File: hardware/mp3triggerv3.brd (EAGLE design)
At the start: 160 x 100 mm, 0 parts

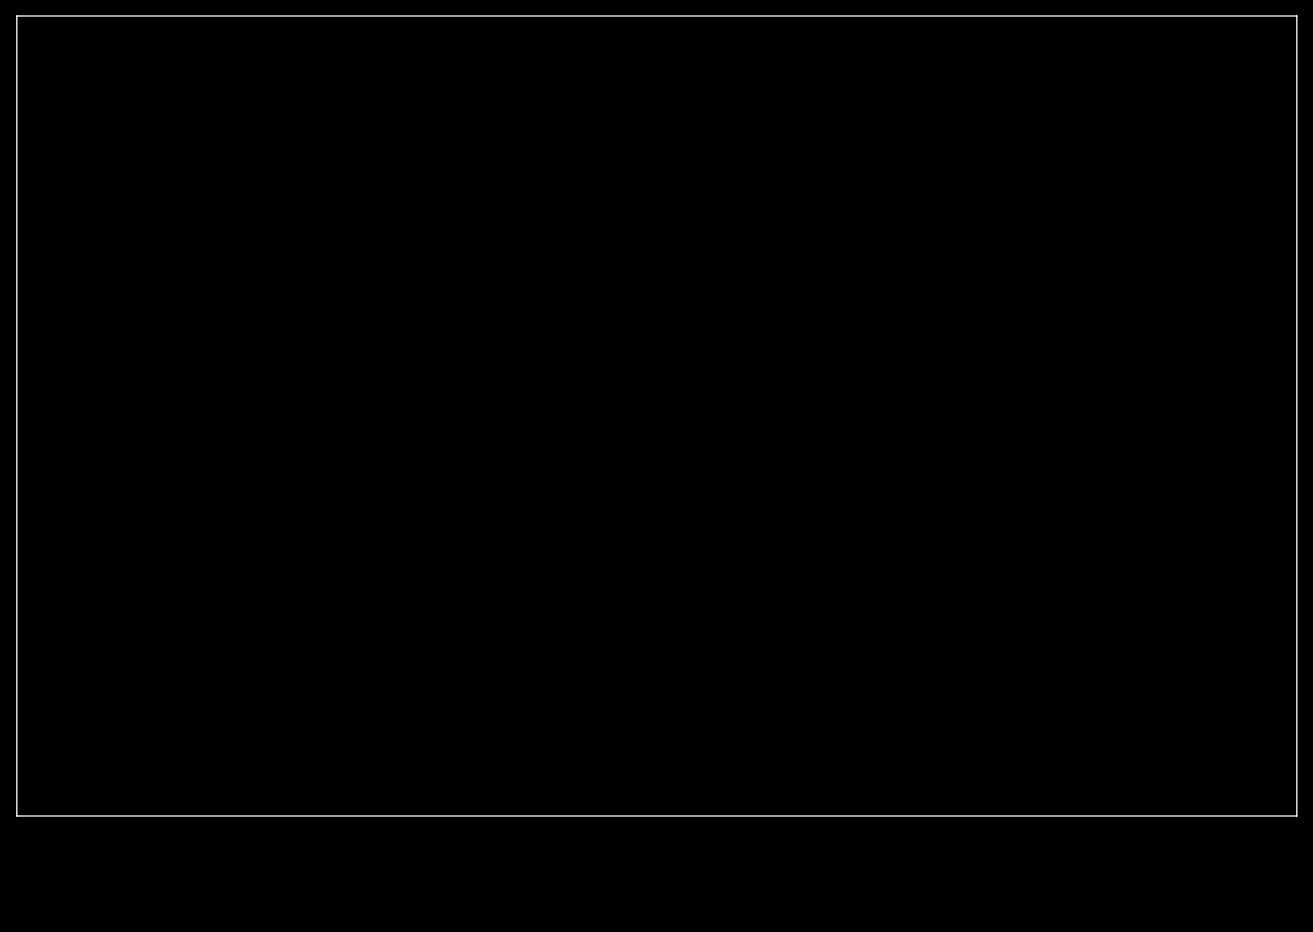
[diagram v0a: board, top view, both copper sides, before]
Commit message: added Jamie's project files
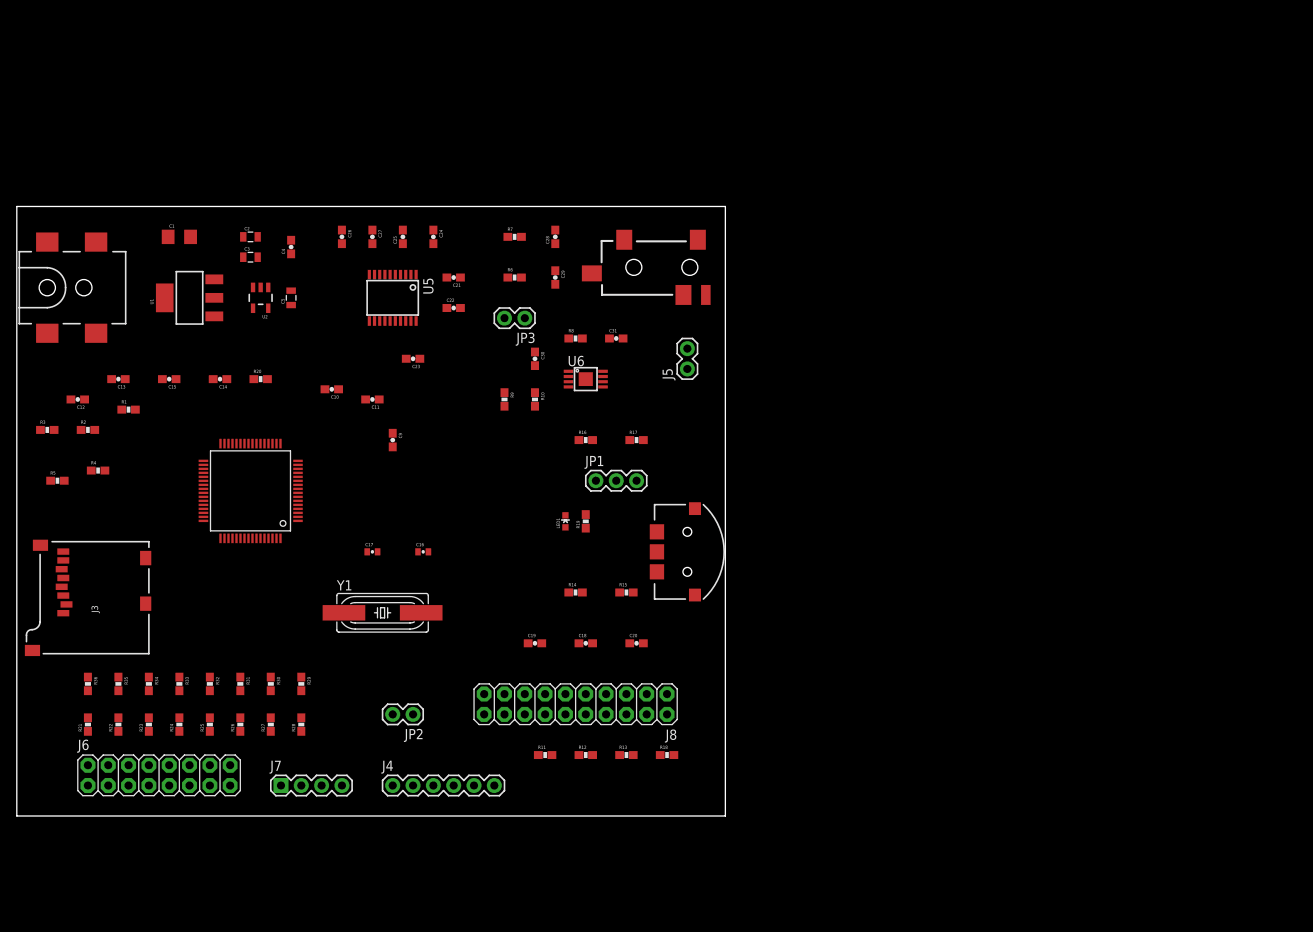
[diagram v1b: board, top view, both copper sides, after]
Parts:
- added C1: 10uF, SparkFun-Capacitors:1206
- added C10, C13, C15, C18, C19, C21, C22, C23, C24, C25, C26, C4, C9: 0.1uF, SparkFun-Capacitors:0603-CAP
- added C11, C30, C31: 1uF, SparkFun-Capacitors:0603-CAP
- added C12: 4.7uF, SparkFun-Capacitors:0603-CAP
- added C14, C20: 2.2uF, SparkFun-Capacitors:0603-CAP
- added C16, C17: 33pF, SparkFun-Capacitors:0402-CAP
- added C2: 10uF, SparkFun-Capacitors:0805
- added C27: 10uF, SparkFun-Capacitors:0603-CAP
- added C28, C29: 2200pF, SparkFun-Capacitors:0603-CAP
- added C3, C5: 2.2uF, SparkFun-Capacitors:0805
- added J1: 5.5x2.1mm Barrel, SparkFun-Connectors:POWER_JACK_SMD
- added J2: (no value), SparkFun-Connectors:AUDIO-JACK-3.5MM-SMD
- added J3: USD-SOCKETNEW, robertsonics:MICRO-SD-SOCKET-PP
- added J4: (no value), SparkFun-Connectors:1X06
- added J5, JP2, JP3: (no value), SparkFun-Connectors:1X02
- added J6: M08X2, SparkFun-Connectors:2X8
- added J7: (no value), SparkFun-Connectors:1X04
- added J8: M10X2, SparkFun-Connectors:2X10
- added JP1: (no value), SparkFun-Connectors:1X03
- added LED1: (no value), SparkFun-LED:LED-0603
- added R1, R2, R3, R4, R5: 47K, SparkFun-Passives:0603-RES
- added R10, R9: 22K, SparkFun-Passives:0603-RES
- added R11, R12, R13, R14, R15, R16, R17, R18, R20, R29, R30, R31, R32, R33, R34, R35, R36, R8: 10K, SparkFun-Passives:0603-RES
- added R19: 330, SparkFun-Passives:0603-RES
- added R21, R22, R23, R24, R25, R26, R27, R28: 100, SparkFun-Passives:0603-RES
- added R6, R7: 470, SparkFun-Passives:0603-RES
- added S1: NAV_SWITCHSMD, SparkFun-Electromechanical:NAV_SWITCH
- added U1: NCP1117, SparkFun-PowerIC:SOT223
- added U2: MIC5323-3.3, SparkFun-PowerIC:SOT23-5
- added U4: STM32F405RG, robertsonics:TQFP-10X10-64
- added U5: PCM5100, robertsonics:PW_R-PDSO-G20
- added U6: LM4990, robertsonics:S-PDSO-G08
- added Y1: 8MHz, SparkFun-FreqCtrl:HC49UP
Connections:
- new net +5V: C2.1, C3.1, C31.2, J7.4, JP2.2, U1.2, U1.4, U2.1, U2.3, U6.6
- new net AMPENA: R8.2, U4.P$11, U6.1
- new net AMPIN: JP3.2, R9.1
- new net BOOT0: JP1.2, U4.P$60
- new net DEMP: U4.P$10, U5.10
- new net FILTER: U4.P$9, U5.11
- new net GND: C1.2, C10.2, C11.2, C12.2, C13.2, C14.2, C15.2, C16.1, C17.1, C18.2, C19.2, C2.2, C20.2, C21.1, C22.2, C23.1, C25.2, C26.1, C27.1, C28.1, C29.1, C3.2, C30.1, C31.1, C4.2, C5.2, J1.GND, J1.P$4, J2.SLEEVE, J3.6, J3.CD2, J3.GND1, J3.GND3, J4.1, J6.1, J6.11, J6.13, J6.15, J6.3, J6.5, J6.7, J6.9, J7.1, J8.10, J8.12, J8.14, J8.16, J8.18, J8.20, J8.4, J8.6, J8.8, R11.1, R12.1, R13.1, R16.2, R20.2, R8.1, S1.C, U1.1, U2.2, U4.P$12, U4.P$18, U4.P$63, U5.16, U5.19, U5.3, U5.9, U6.7
- new net I2S_BCLK: U4.P$34, U5.13
- new net I2S_DOUT: U4.P$36, U5.14
- new net I2S_LRCK: U4.P$33, U5.15
- new net I2S_MCLK: U4.P$37, U5.12
- new net JTCK: J8.9, U4.P$49
- new net JTDI: J8.5, U4.P$50
- new net JTDO: J8.13, U4.P$55
- new net JTMS: J8.7, U4.P$46
- new net JTRST: J8.3, U4.P$56
- new net LED1: LED1.C, U4.P$24
- new net LOUTL: C28.2, J2.TIP, JP3.1, R7.2
- new net LOUTR: C29.2, J2.RING, R6.2
- new net MUTE: U4.P$8, U5.17
- new net N$10: JP1.3, R17.2
- new net N$11: LED1.A, R19.2
- new net N$12: R20.1, U4.P$28
- new net N$13: J8.19, R11.2
- new net N$14: C23.2, U5.18
- new net N$15: R6.1, U5.7
- new net N$16: C24.2, U5.2
- new net N$17: C24.1, U5.4
- new net N$18: C25.1, U5.5
- new net N$19: R7.1, U5.6
- new net N$2: C4.1, U2.4
- new net N$20: C30.2, U6.2, U6.3
- new net N$21: J8.17, R12.2
- new net N$22: J8.11, R13.2
- new net N$23: J6.2, R21.1, R36.1
- new net N$24: J6.4, R22.1, R35.1
- new net N$25: J6.6, R23.1, R34.1
- new net N$26: J6.8, R24.1, R33.1
- new net N$27: J6.10, R25.1, R32.1
- new net N$28: J6.12, R26.1, R31.1
- new net N$29: R10.1, R9.2, U6.4
- new net N$3: C9.2, U4.P$1
- new net N$30: J6.14, R27.1, R30.1
- new net N$31: J6.16, R28.1, R29.1
- new net N$32: J4.3, JP2.1
- new net N$4: C14.1, U4.P$31
- new net N$5: C16.2, U4.P$5, Y1.2
- new net N$6: C17.2, U4.P$6, Y1.1
- new net N$7: JP1.1, R16.1
- new net N$8: C20.1, U4.P$47
- new net N$9: J4.4, R15.2
- new net NAV1: S1.1, U4.P$2
- new net NAV2: S1.2, U4.P$4
- new net NAVT: S1.T, U4.P$3
- new net NRST: J8.15, R18.1, U4.P$7
- new net PLAYOUT: J7.2, U4.P$25
- new net RXD: R14.1, R15.1, U4.P$43
- new net SD_CD: J3.CD1, U4.P$26
- new net SD_CK: J3.5, U4.P$53
- new net SD_CMD: J3.3, R3.1, U4.P$54
- new net SD_D0: J3.7, R2.1, U4.P$39
- new net SD_D1: J3.8, R1.1, U4.P$40
- new net SD_D2: J3.1, R5.1, U4.P$51
- new net SD_D3: J3.2, R4.1, U4.P$52
- new net SPKR+: J5.2, U6.8
- new net SPKR-: J5.1, R10.2, U6.5
- new net TRIG00: R21.2, U4.P$14
- new net TRIG01: R22.2, U4.P$15
- new net TRIG02: R23.2, U4.P$16
- new net TRIG03: R24.2, U4.P$17
- new net TRIG04: R25.2, U4.P$20
- new net TRIG05: R26.2, U4.P$21
- new net TRIG06: R27.2, U4.P$22
- new net TRIG07: R28.2, U4.P$23
- new net TXD: J4.5, U4.P$42
- new net VCC: C10.1, C11.1, C12.1, C13.1, C15.1, C18.1, C19.1, C21.2, C22.1, C26.2, C27.2, C5.1, C9.1, J3.4, J7.3, J8.1, J8.2, R1.2, R14.2, R17.1, R18.2, R19.1, R2.2, R29.2, R3.2, R30.2, R31.2, R32.2, R33.2, R34.2, R35.2, R36.2, R4.2, R5.2, U2.5, U4.P$13, U4.P$19, U4.P$32, U4.P$48, U4.P$64, U5.1, U5.20, U5.8
- new net VIN_9V: C1.1, J1.VIN0, U1.3
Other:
- board size 160 x 100 mm -> 88.6 x 76.2 mm

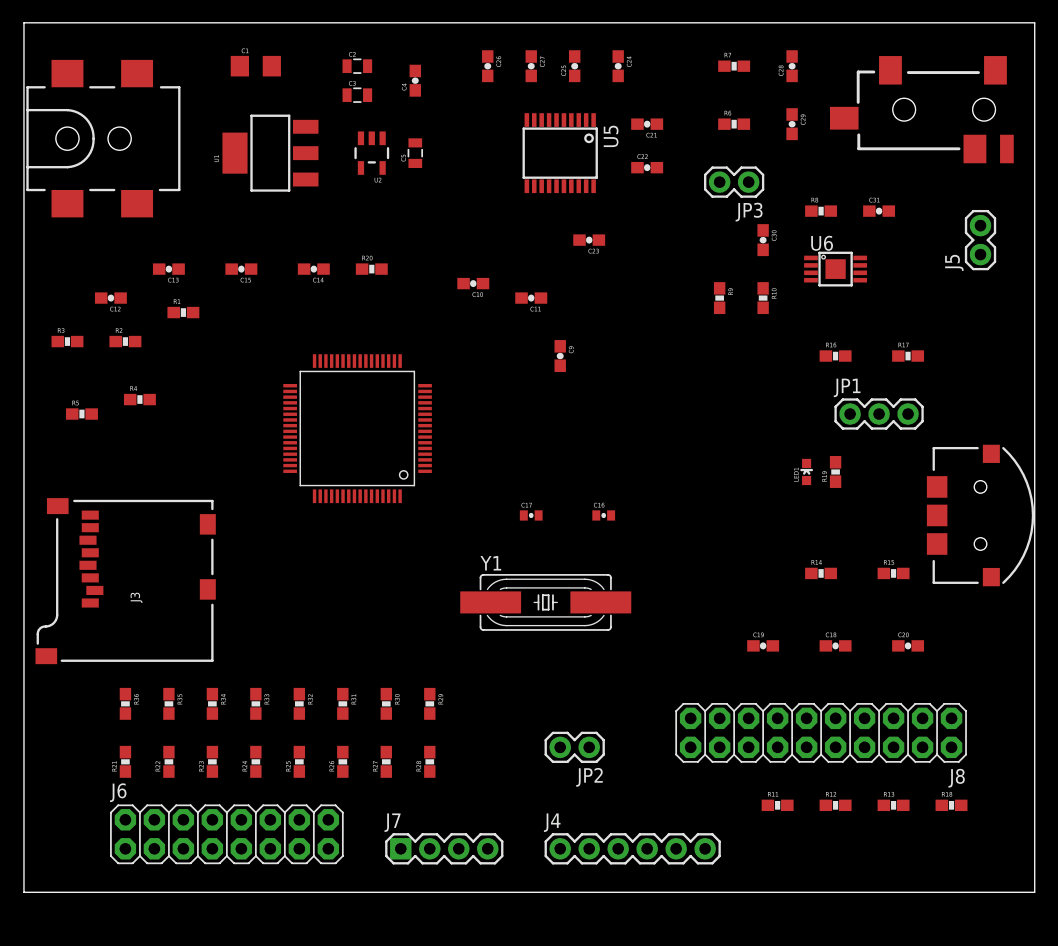
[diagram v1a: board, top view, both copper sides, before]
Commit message: v010
files sent to Jamie
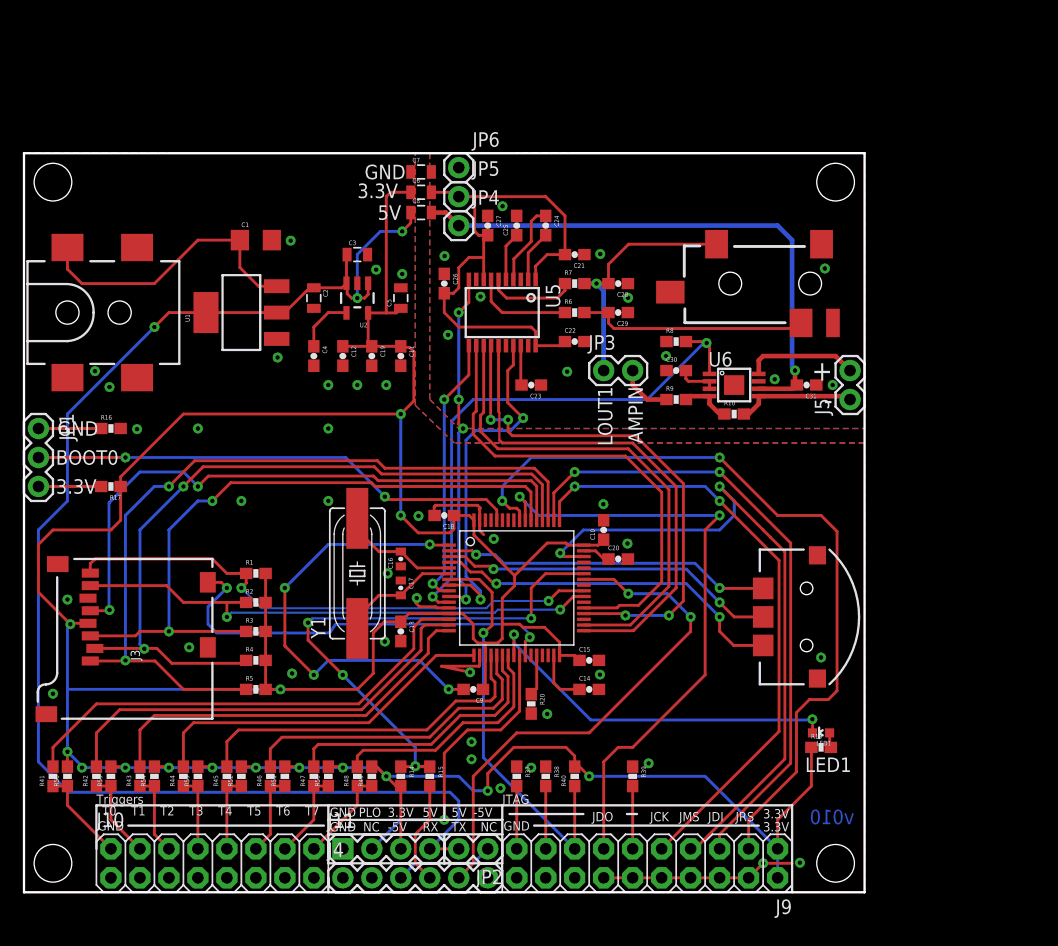
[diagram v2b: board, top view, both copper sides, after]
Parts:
- removed J6: M08X2, SparkFun-Connectors:2X8
- removed J7: (no value), SparkFun-Connectors:1X04
- removed J8: M10X2, SparkFun-Connectors:2X10
- removed R11, R12, R13, R18, R29, R30, R31, R32, R33, R34, R35, R36: 10K, SparkFun-Passives:0603-RES
- removed R21, R22, R23, R24, R25, R26, R27, R28: 100, SparkFun-Passives:0603-RES
- added C6: 3.3V jumper, SparkFun-Capacitors:0805
- added C7: GND jumper, SparkFun-Capacitors:0805
- added C8: 5V jumper, SparkFun-Capacitors:0805
- added J10: M08X2, SparkFun-Connectors:2X8
- added J11: (no value), SparkFun-Connectors:1X04
- added J9: M10X2, SparkFun-Connectors:2X10
- added JP4, JP5, JP6: M01PTH, SparkFun-Connectors:1X01
- added R37, R38, R39, R40, R49, R50, R51, R52, R53, R54, R55, R56: 10K, SparkFun-Passives:0603-RES
- added R41, R42, R43, R44, R45, R46, R47, R48: 100, SparkFun-Passives:0603-RES
- added STANDOFF1, STANDOFF2, STANDOFF3, STANDOFF4: STAND-OFF, SparkFun-Electromechanical:STAND-OFF
- moved JP1 71.1 mm to (1.27, 40.6), turned to 270 degrees
- moved R17 70.8 mm to (7.62, 35.6), turned to 180 degrees
- moved R16 63.8 mm to (7.62, 40.6)
- moved C15 45.9 mm to (49.5, 20.3), turned to 0 degrees
- moved R15 44.4 mm to (35.6, 10.2), turned to 270 degrees
- moved C14 44.0 mm to (49.5, 17.8), turned to 0 degrees
- moved C19 42.7 mm to (30.5, 47.0), turned to 270 degrees
- moved R14 40.9 mm to (33.0, 10.2), turned to 270 degrees
- moved R20 40.6 mm to (44.5, 16.5), turned to 270 degrees
- moved C13 37.7 mm to (33.0, 22.9), turned to 270 degrees
- moved C18 36.1 mm to (36.8, 33.0), turned to 180 degrees
- moved R3 30.3 mm to (20.3, 22.9)
- moved C9 30.2 mm to (39.4, 17.8), turned to 180 degrees
- moved R5 28.5 mm to (20.3, 17.8)
- moved C20 26.5 mm to (52.1, 29.2)
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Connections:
- removed net N$13: J8.19, R11.2
- removed net N$21: J8.17, R12.2
- removed net N$22: J8.11, R13.2
- removed net N$23: J6.2, R21.1, R36.1
- removed net N$24: J6.4, R22.1, R35.1
- removed net N$25: J6.6, R23.1, R34.1
- removed net N$26: J6.8, R24.1, R33.1
- removed net N$27: J6.10, R25.1, R32.1
- removed net N$28: J6.12, R26.1, R31.1
- removed net N$30: J6.14, R27.1, R30.1
- removed net N$31: J6.16, R28.1, R29.1
- new net N$1: J9.19, R37.2
- new net N$33: J9.17, R38.2
- new net N$34: J9.11, R39.2
- new net N$35: J10.2, R41.1, R56.1
- new net N$36: J10.4, R42.1, R55.1
- new net N$37: J10.6, R43.1, R54.1
- new net N$38: J10.8, R44.1, R53.1
- new net N$39: J10.10, R45.1, R52.1
- new net N$40: J10.12, R46.1, R51.1
- new net N$41: J10.14, R47.1, R50.1
- new net N$42: J10.16, R48.1, R49.1
- net +5V: now also C8.1, C8.2, J11.4, JP4.1; no longer J7.4
- net GND: now also C7.1, C7.2, J10.1, J10.11, J10.13, J10.15, J10.3, J10.5, J10.7, J10.9, J11.1, J9.10, J9.12, J9.14, J9.16, J9.18, J9.20, J9.4, J9.6, J9.8, JP6.1, R37.1, R38.1, R39.1; no longer J6.1, J6.11, J6.13, J6.15, J6.3, J6.5, J6.7, J6.9, J7.1, J8.10, J8.12, J8.14, J8.16, J8.18, J8.20, J8.4, J8.6, J8.8, R11.1, R12.1, R13.1
- net JTCK: now also J9.9; no longer J8.9
- net JTDI: now also J9.5; no longer J8.5
- net JTDO: now also J9.13; no longer J8.13
- net JTMS: now also J9.7; no longer J8.7
- net JTRST: now also J9.3; no longer J8.3
- net NRST: now also J9.15, R40.1; no longer J8.15, R18.1
- net PLAYOUT: now also J11.2; no longer J7.2
- net TRIG00: now also R41.2; no longer R21.2
- net TRIG01: now also R42.2; no longer R22.2
- net TRIG02: now also R43.2; no longer R23.2
- net TRIG03: now also R44.2; no longer R24.2
- net TRIG04: now also R45.2; no longer R25.2
- net TRIG05: now also R46.2; no longer R26.2
- net TRIG06: now also R47.2; no longer R27.2
- net TRIG07: now also R48.2; no longer R28.2
- net VCC: now also C6.1, C6.2, J11.3, J9.1, J9.2, JP5.1, R40.2, R49.2, R50.2, R51.2, R52.2, R53.2, R54.2, R55.2, R56.2; no longer J7.3, J8.1, J8.2, R18.2, R29.2, R30.2, R31.2, R32.2, R33.2, R34.2, R35.2, R36.2
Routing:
- net VCC: track 0.00 -> 349.2 mm, vias 0 -> 15
- net +5V: track 0.00 -> 173.0 mm, vias 0 -> 4
- net SD_D2: track 0.00 -> 70.6 mm, vias 0 -> 2
- net JTRST: track 0.00 -> 69.0 mm, vias 0 -> 2
- net SD_D3: track 0.00 -> 65.8 mm, vias 0 -> 2
- net JTMS: track 0.00 -> 59.6 mm, vias 0 -> 2
- net SD_CMD: track 0.00 -> 59.0 mm, vias 0 -> 2
- net JTDI: track 0.00 -> 55.9 mm, vias 0 -> 2
- net JTDO: track 0.00 -> 54.6 mm, vias 0 -> 2
- net SD_CK: track 0.00 -> 54.0 mm, vias 0 -> 2
- net JTCK: track 0.00 -> 53.6 mm, vias 0 -> 2
- net SD_D1: track 0.00 -> 48.0 mm, vias 0 -> 2
- net RXD: track 0.00 -> 47.8 mm, vias 0 -> 4
- net SD_D0: track 0.00 -> 47.6 mm, vias 0 -> 2
- net AMPENA: track 0.00 -> 47.6 mm, vias 0 -> 2
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- added copper zone on layer 1, net GND
- added copper zone on layer 16, net GND
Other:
- board size 88.6 x 76.2 mm -> 73.7 x 64.8 mm
- board text added: "+"
- board text added: "-"
- board text added: "-5V"
- board text added: "3.3V"
- board text added: "5V"
- board text added: "AMPIN"
- board text added: "BOOT0"
- board text added: "GND"
- board text added: "JCK"
- board text added: "JDI"
- board text added: "JDO"
- board text added: "JMS"
- board text added: "JRS"
- board text added: "JTAG"
- board text added: "LED1"
- board text added: "LOUT1"
- board text added: "NC"
- board text added: "PLO"
- board text added: "RX"
- board text added: "T0"
- board text added: "T1"
- board text added: "T2"
- board text added: "T3"
- board text added: "T4"
- board text added: "T5"
- board text added: "T6"
- board text added: "T7"
- board text added: "TX"
- board text added: "Triggers"
- board text added: "v010"
